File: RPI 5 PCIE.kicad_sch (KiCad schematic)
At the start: 1 part, among them J1 Conn_01x16

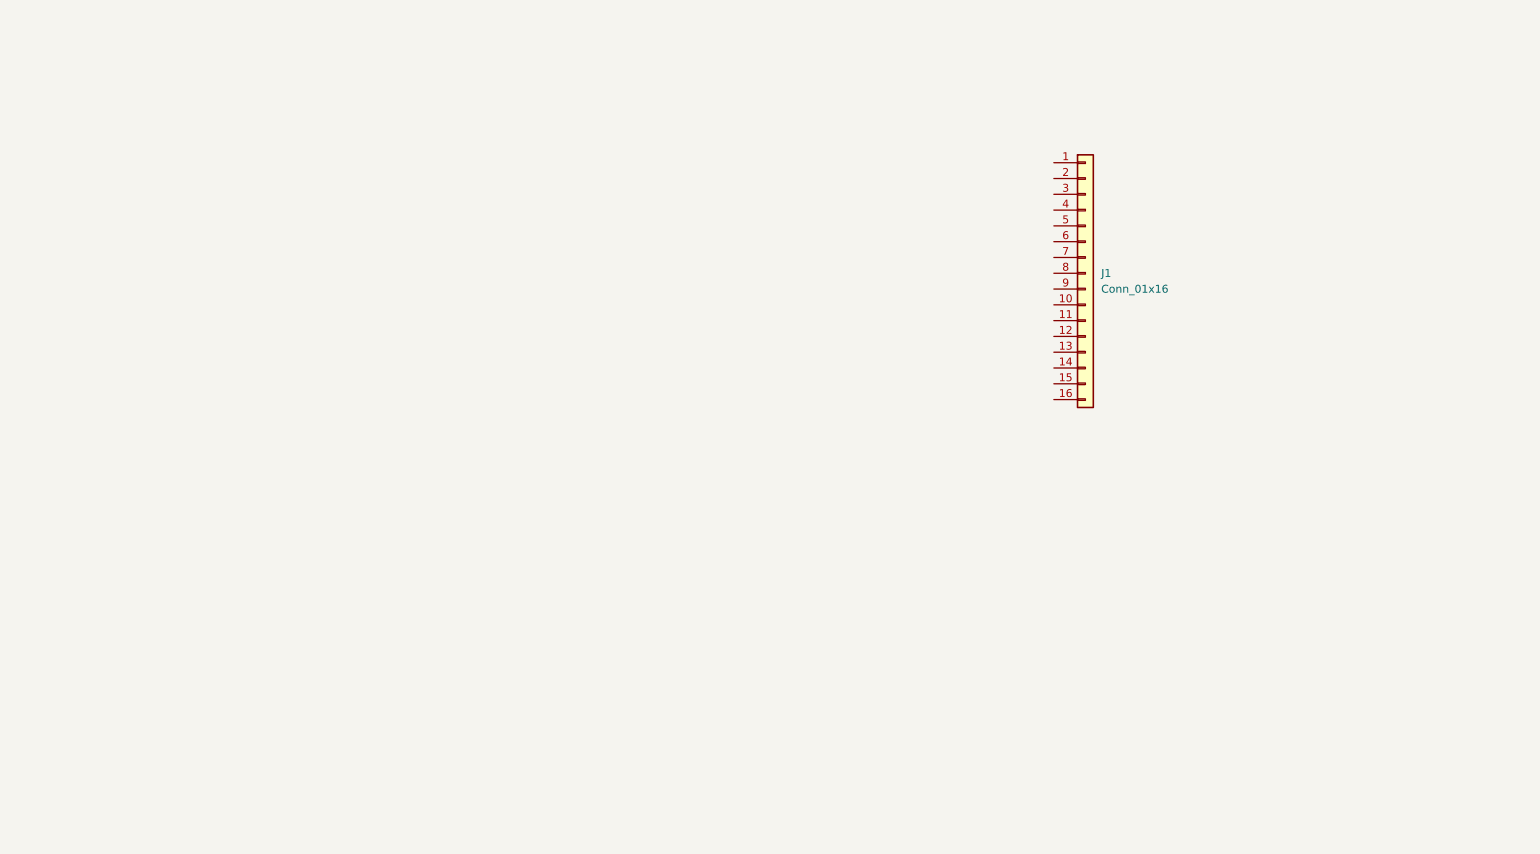
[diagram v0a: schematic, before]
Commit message: Created Schematic
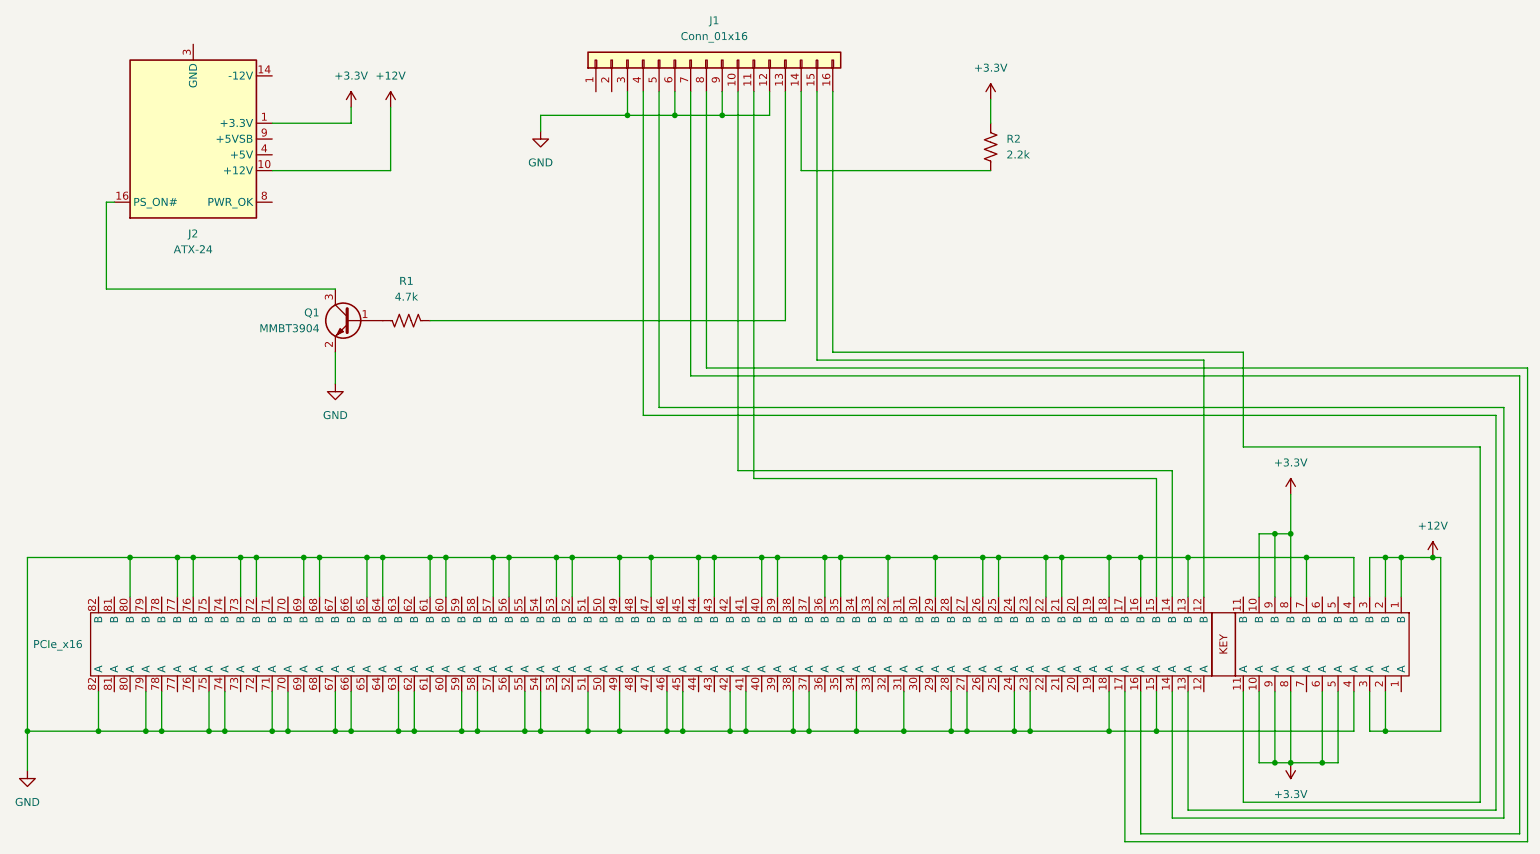
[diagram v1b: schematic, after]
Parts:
- added J2: ATX-24, symbol Connector:ATX-24
- added PCIe_x16: ~, symbol PCIE:PCIE_x16_Unamed_Pins
- added Q1: MMBT3904, Package_TO_SOT_SMD:SOT-23, symbol Transistor_BJT:MMBT3904
- added R1: 4.7k, symbol Device:R_US
- added R2: 2.2k, symbol Device:R_US
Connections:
- net at J1.10 (Pin_10): now also PCIe_x16.14 (B)
- net at J1.11 (Pin_11): now also PCIe_x16.15 (B)
- net GND: now reaches J1.12 (Pin_12)
- net GND: now also J1.3 (Pin_3), J1.6 (Pin_6), J1.9 (Pin_9), PCIe_x16.13 (B), PCIe_x16.15 (B), PCIe_x16.16 (B), PCIe_x16.18 (B), PCIe_x16.21 (B), PCIe_x16.22 (B), PCIe_x16.23 (B), PCIe_x16.24 (B), PCIe_x16.25 (B), PCIe_x16.26 (B), PCIe_x16.27 (B), PCIe_x16.28 (B), PCIe_x16.29 (B), PCIe_x16.31 (B), PCIe_x16.32 (B), PCIe_x16.34 (B), PCIe_x16.35 (B), PCIe_x16.36 (B), PCIe_x16.37 (B), PCIe_x16.38 (B), PCIe_x16.39 (B), PCIe_x16.4 (B), PCIe_x16.40 (B), PCIe_x16.41 (B), PCIe_x16.42 (B), PCIe_x16.43 (B), PCIe_x16.44 (B), PCIe_x16.45 (B), PCIe_x16.46 (B), PCIe_x16.47 (B), PCIe_x16.49 (B), PCIe_x16.51 (B), PCIe_x16.52 (B), PCIe_x16.53 (B), PCIe_x16.54 (B), PCIe_x16.55 (B), PCIe_x16.56 (B), PCIe_x16.57 (B), PCIe_x16.58 (B), PCIe_x16.59 (B), PCIe_x16.60 (B), PCIe_x16.61 (B), PCIe_x16.62 (B), PCIe_x16.63 (B), PCIe_x16.64 (B), PCIe_x16.65 (B), PCIe_x16.66 (B), PCIe_x16.67 (B), PCIe_x16.68 (B), PCIe_x16.69 (B), PCIe_x16.7 (B), PCIe_x16.70 (B), PCIe_x16.71 (B), PCIe_x16.72 (B), PCIe_x16.73 (B), PCIe_x16.74 (B), PCIe_x16.75 (B), PCIe_x16.76 (B), PCIe_x16.77 (B), PCIe_x16.78 (B), PCIe_x16.79 (B), PCIe_x16.80 (B), PCIe_x16.82 (B), Q1.2 (E)
- net at J1.13 (Pin_13): now also R1.1
- net at J1.14 (Pin_14): now also R2.2
- net at J1.15 (Pin_15): now also PCIe_x16.12 (B)
- net at J1.16 (Pin_16): now also PCIe_x16.11 (B)
- net at J1.4 (Pin_4): now also PCIe_x16.13 (B)
- net at J1.5 (Pin_5): now also PCIe_x16.14 (B)
- net at J1.7 (Pin_7): now also PCIe_x16.16 (B)
- net at J1.8 (Pin_8): now also PCIe_x16.17 (B)
- new net: Q1.1 (B), R1.2
- new net: J2.16 (PS_ON#), Q1.3 (C)
- new net: J2.15 (GND), J2.17 (GND), J2.18 (GND), J2.19 (GND), J2.24 (GND), J2.3 (GND), J2.5 (GND), J2.7 (GND)
- new net: J2.21 (+5V), J2.22 (+5V), J2.23 (+5V), J2.4 (+5V), J2.6 (+5V)
- new net +12V: J2.10 (+12V), J2.11 (+12V), PCIe_x16.1 (B), PCIe_x16.2 (B), PCIe_x16.3 (B)
- new net +3.3V: J2.1 (+3.3V), J2.12 (+3.3V), J2.13 (+3.3V), J2.2 (+3.3V), PCIe_x16.10 (B), PCIe_x16.5 (B), PCIe_x16.6 (B), PCIe_x16.8 (B), PCIe_x16.9 (B), R2.1
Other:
- moved on the sheet: J1
